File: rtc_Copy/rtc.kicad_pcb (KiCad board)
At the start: 2 copper layers, 23.5 x 32.4 mm, 17 parts, among them J1 Conn_02x03_Odd_Even, J2 Conn_01x04, J3 Conn_01x04, J4 Conn_01x04, U1 PCF8563T/5_518, Y1 LFXTAL016178REEL

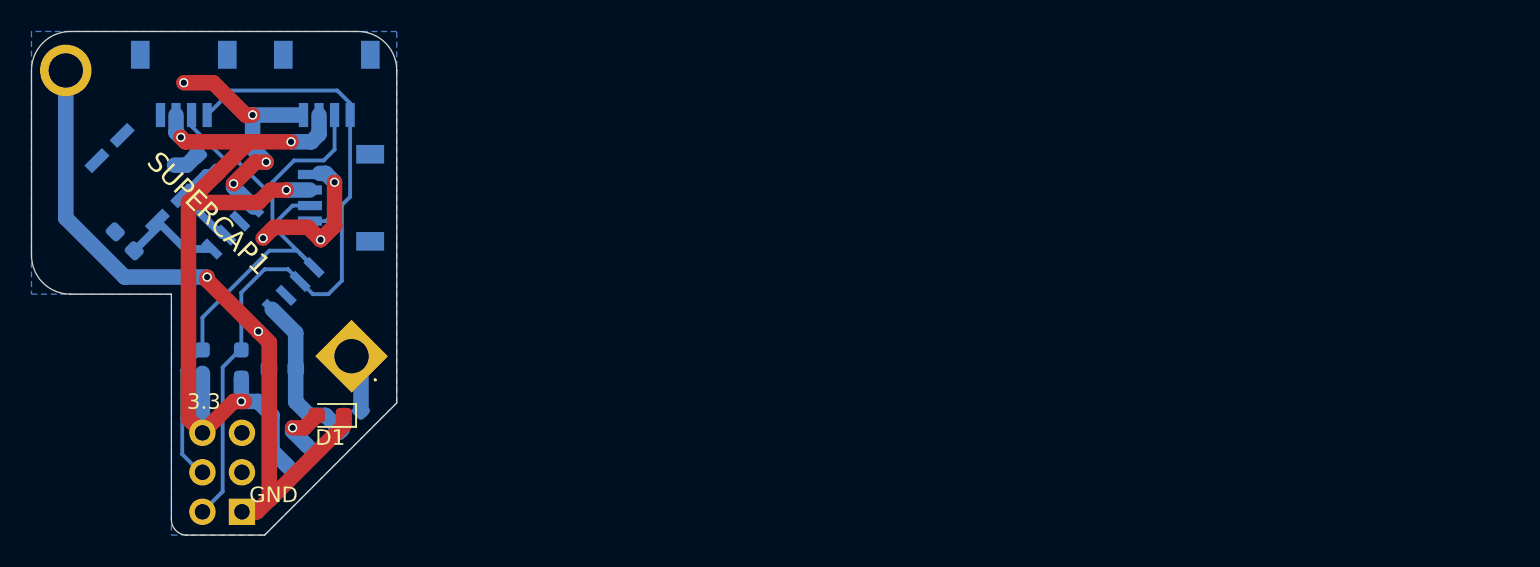
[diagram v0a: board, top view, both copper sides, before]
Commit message: new rtc
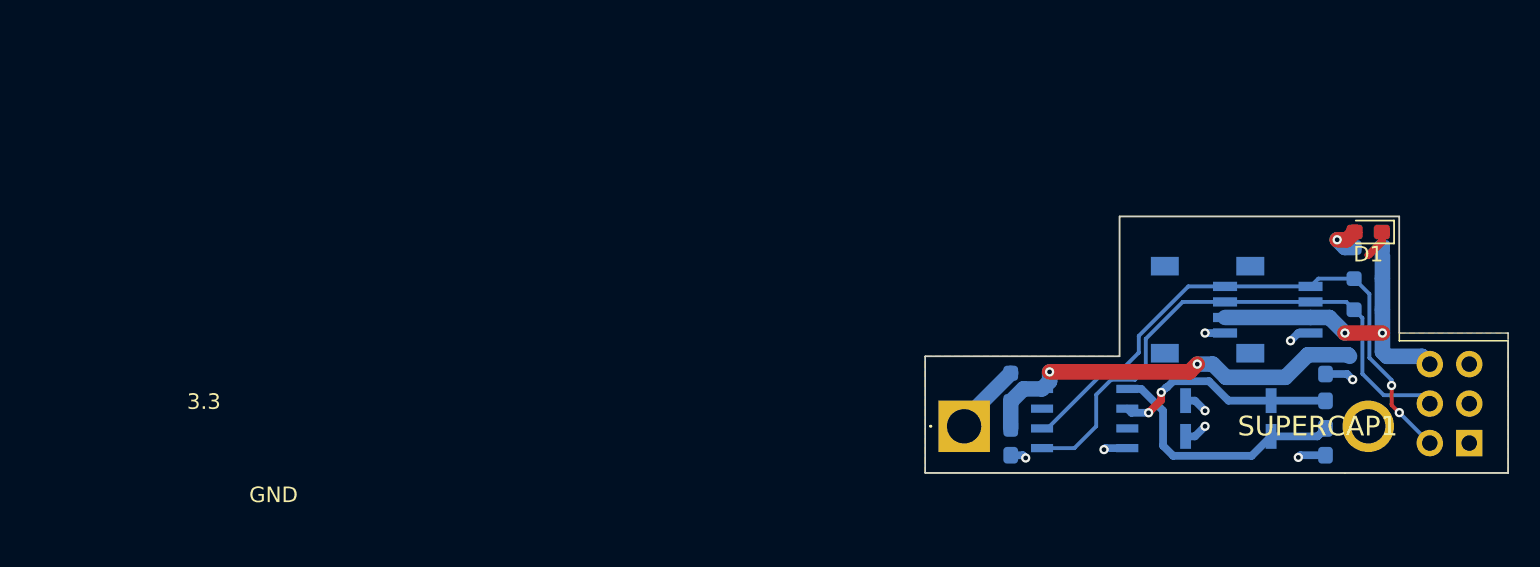
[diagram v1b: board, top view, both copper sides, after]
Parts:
- removed J4: Conn_01x04, pcb_footprints:SM04BSRSSTB
- moved J1 79.1 mm to (233.5, 94.1)
- moved C1 78.3 mm to (224.2, 94.0), turned to -90 degrees
- moved R2 75.1 mm to (227.0, 85.5), turned to 0 degrees
- moved C3 73.4 mm to (224.2, 90.5), turned to 90 degrees
- moved R3 72.7 mm to (227.0, 83.5), turned to 0 degrees
- moved Y1 71.7 mm to (218.0, 92.5), turned to 180 degrees
- moved G*** 70.8 mm to (214.0, 82.5), turned to 180 degrees
- moved R4 70.2 mm to (227.0, 81.5), turned to 180 degrees
- moved D2 69.4 mm to (227.0, 88.5), turned to 0 degrees
- moved D1 67.8 mm to (227.0, 80.5)
- moved J3 60.2 mm to (221.0, 85.5), turned to 90 degrees
- moved J2 57.4 mm to (215.5, 85.5), turned to 90 degrees
- moved U1 53.9 mm to (208.8, 92.5), turned to 180 degrees
- moved C2 47.1 mm to (204.0, 94.0), turned to -90 degrees
- moved R1 42.5 mm to (204.0, 90.5), turned to -90 degrees
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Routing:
- net GND: track 76.1 -> 14.0 mm, vias 9 -> 8
- net +3.3V: track 55.8 -> 20.1 mm, vias 4 -> 2
- net Net-(D2-K): track 10.3 -> 25.9 mm, vias 0 -> 2
- net scl: track 48.3 -> 37.5 mm, vias 0 -> 2
- net Net-(U1-OSCI): track 6.78 -> 16.6 mm
- net sda: track 45.3 -> 36.0 mm
- net Net-(U1-OSCO): track 6.47 -> 14.5 mm, vias 0 -> 2
- net Net-(SUPERCAP1-+): track 3.76 -> 4.66 mm
- net Net-(D1-A): track 3.43 -> 2.63 mm
- added copper zone on F.Cu, net GND
- removed copper zone on B.Cu, net GND
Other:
- board size 23.5 x 32.4 mm -> 37.5 x 16.5 mm
- board text added: "Made by Hailin Chen"
- board text removed: "Designed by A. Ai"
